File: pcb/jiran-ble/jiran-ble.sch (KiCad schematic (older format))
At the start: 165 parts, among them J1 BATT, J2 USB-C Conn, J3 SWD, J4 BATT, J5 USB-C Conn, J6 SWD, Q1 AO3407, Q3 AO3407, SW1 SW_PUSH, SW10 SW_Push, SW11 SW_Push, SW12 SW_Push, SW13 SW_Push, SW14 SW_Push, SW15 SW_Push, SW16 SW_Push, SW17 SW_Push, SW18 SW_Push, SW19 SW_Push, SW2 SW_Push, SW20 SW_Push, SW21 SW_Push, SW22 SW_Push, SW23 SW_Push, SW24 SW_Push, SW25 SW_Push, SW26 SW_Push, SW27 SW_Push, SW28 SW_Push, SW29 SW_Push, SW3 SW_Push, SW30 SW_PUSH, SW31 SW_Push, SW32 SW_Push, SW33 SW_Push, SW34 SW_Push, SW35 SW_Push, SW36 SW_Push, SW37 SW_Push, SW38 SW_Push, SW39 SW_Push, SW4 SW_Push, SW40 SW_Push, SW41 SW_Push, SW42 SW_Push, SW43 SW_Push, SW44 SW_Push, SW45 SW_Push, SW46 SW_Push, SW47 SW_Push, SW48 SW_Push, SW49 SW_Push, SW5 SW_Push, SW50 SW_Push, SW51 SW_Push, SW52 SW_Push, SW53 SW_Push, SW54 SW_Push, SW55 SW_Push, SW56 SW_Push, SW57 SW_Push, SW58 SW_Push, SW6 SW_Push, SW7 SW_Push, SW8 SW_Push, SW9 SW_Push, U1 XC6220B331MR-G, U3 TP4054, U4 XC6220B331MR-G, U5 E73-2G4M08S1C, U6 TP4054, X2 Crystal

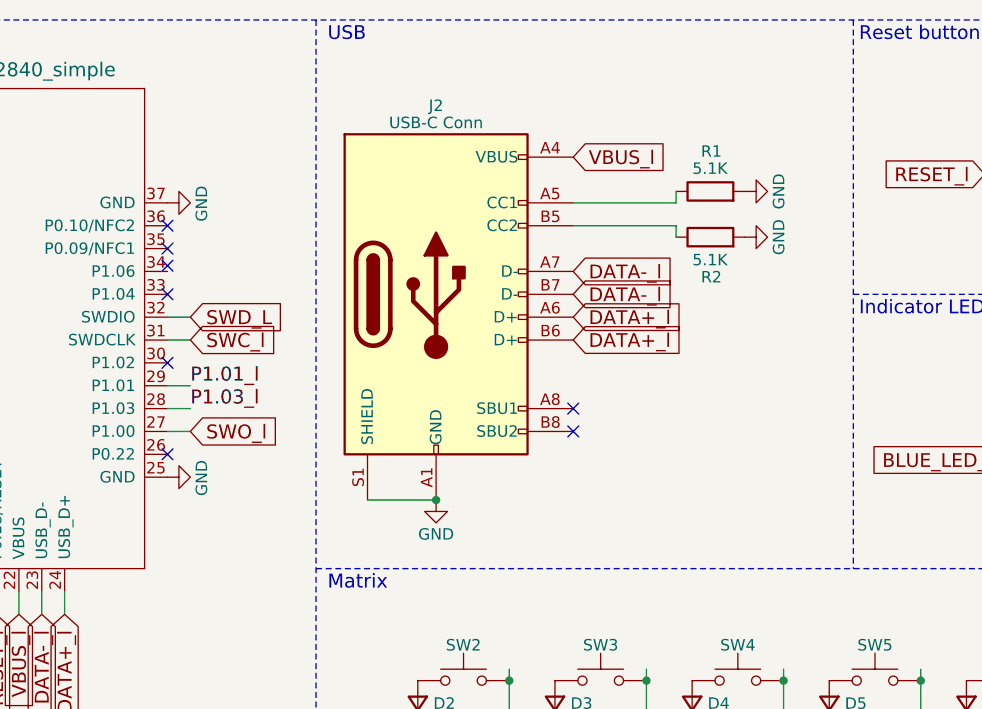
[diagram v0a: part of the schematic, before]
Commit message: USB circuit is now simpler
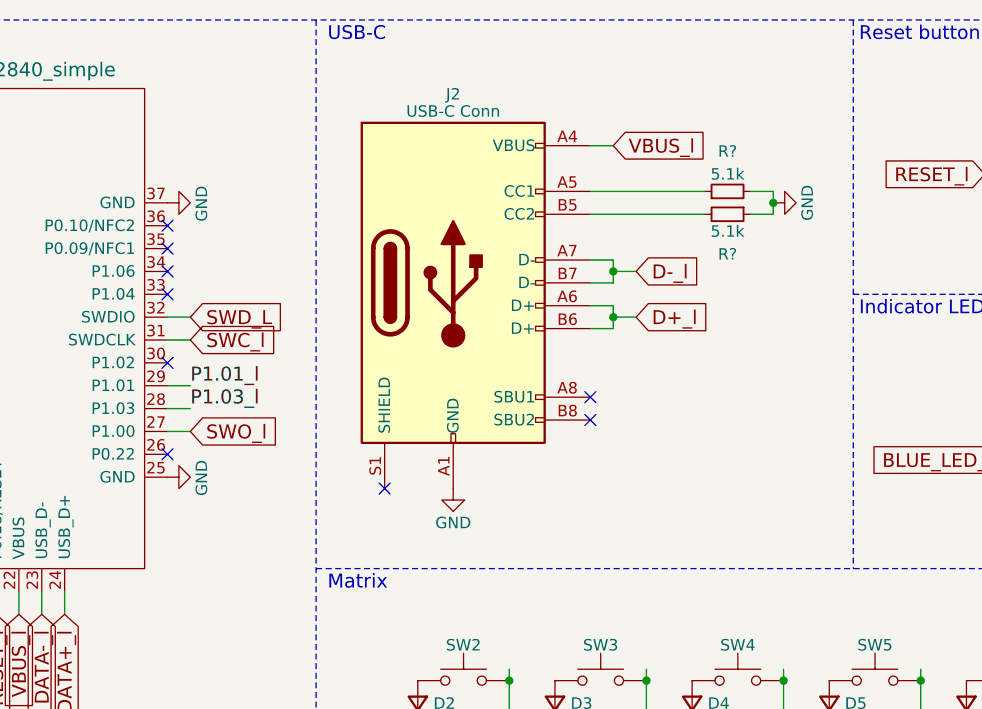
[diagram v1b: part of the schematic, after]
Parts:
- removed R1, R2: 5.1K, jiran-ble:Resistor_SMD_0805, symbol Device:R
- added R? (x2): 5.1k, symbol Device:R_Small
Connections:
- net labels added: D+_l, D-_l
- wire segments 233 -> 245
- no-connect marks 30 -> 31
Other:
- note added: "USB-C"
- moved on the sheet: J2
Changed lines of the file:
@@
 NRF52840
 Text Notes 4100 600  0    60   ~ 0
-USB
+USB-C
 Text Notes 6425 1800 0    60   ~ 0
 Indicator LED
@@
 Text Notes 15415 11075 0    70   ~ 14
 r0.2
-Text GLabel 5175 1600 2    60   Input ~ 0
-DATA-_l
-$Comp
-L Device:R R2
-U 1 1 5CAA680B
-P 5775 1450
-F 0 "R2" V 5600 1400 50  0000 L CNN
-F 1 "5.1K" V 5675 1375 50  0000 L CNN
-F 2 "jiran-ble:Resistor_SMD_0805" V 5705 1450 50  0001 C CNN
-F 3 "~" H 5775 1450 50  0001 C CNN
-	1    5775 1450
-	0    -1   -1   0
-$EndComp
-$Comp
-L Device:R R1
-U 1 1 5CAA879F
-P 5775 1250
-F 0 "R1" V 5950 1200 50  0000 L CNN
-F 1 "5.1K" V 5875 1175 50  0000 L CNN
-F 2 "jiran-ble:Resistor_SMD_0805" V 5705 1250 50  0001 C CNN
-F 3 "~" H 5775 1250 50  0001 C CNN
-	1    5775 1250
-	0    -1   -1   0
-$EndComp
-Text GLabel 5175 1700 2    60   Input ~ 0
-DATA-_l
-Text GLabel 5175 1800 2    60   Input ~ 0
-DATA+_l
-Text GLabel 5175 1900 2    60   Input ~ 0
-DATA+_l
 $Comp
 L power:GND #PWR04
 U 1 1 5E5DBB46
-P 5925 1250
-F 0 "#PWR04" H 5925 1000 50  0001 C CNN
-F 1 "GND" H 5925 1100 50  0000 C CNN
-F 2 "" H 5925 1250 50  0001 C CNN
-F 3 "" H 5925 1250 50  0001 C CNN
-	1    5925 1250
-	0    -1   -1   0
-$EndComp
-$Comp
-L power:GND #PWR06
-U 1 1 5E5DDBCF
-P 5925 1450
-F 0 "#PWR06" H 5925 1200 50  0001 C CNN
-F 1 "GND" H 5925 1300 50  0000 C CNN
-F 2 "" H 5925 1450 50  0001 C CNN
-F 3 "" H 5925 1450 50  0001 C CNN
-	1    5925 1450
+P 6050 1300
+F 0 "#PWR04" H 6050 1050 50  0001 C CNN
+F 1 "GND" H 6050 1150 50  0000 C CNN
+F 2 "" H 6050 1300 50  0001 C CNN
+F 3 "" H 6050 1300 50  0001 C CNN
+	1    6050 1300
 	0    -1   -1   0
 $EndComp
@@
 L power:GND #PWR013
 U 1 1 5E5EC00A
-P 4575 2600
-F 0 "#PWR013" H 4575 2350 50  0001 C CNN
-F 1 "GND" H 4575 2450 50  0000 C CNN
-F 2 "" H 4575 2600 50  0001 C CNN
-F 3 "" H 4575 2600 50  0001 C CNN
-	1    4575 2600
+P 4650 2550
+F 0 "#PWR013" H 4650 2300 50  0001 C CNN
+F 1 "GND" H 4650 2400 50  0000 C CNN
+F 2 "" H 4650 2550 50  0001 C CNN
+F 3 "" H 4650 2550 50  0001 C CNN
+	1    4650 2550
 	1    0    0    -1
 $EndComp
-Text GLabel 5175 1100 2    60   Input ~ 0
+Text GLabel 5350 1050 2    60   Input ~ 0
 VBUS_l
 $Comp
 L nrfmicro-rescue:USB_C_Receptacle_USB2.0-Connector J2
 U 1 1 5C743564
-P 4575 1700
-F 0 "J2" H 4575 2525 50  0000 C CNN
-F 1 "USB-C Conn" H 4575 2450 50  0000 C CNN
-F 2 "jiran-ble:USB-C_MidMount" H 4682 2475 50  0001 C CNN
-F 3 "https://www.usb.org/sites/default/files/documents/usb_type-c.zip" H 4725 1700 50  0001 C CNN
-	1    4575 1700
+P 4650 1650
+F 0 "J2" H 4650 2475 50  0000 C CNN
+F 1 "USB-C Conn" H 4650 2400 50  0000 C CNN
+F 2 "jiran-ble:USB-C_MidMount" H 4757 2425 50  0001 C CNN
+F 3 "https://www.usb.org/sites/default/files/documents/usb_type-c.zip" H 4800 1650 50  0001 C CNN
+	1    4650 1650
 	1    0    0    -1
 $EndComp
@@
 Connection ~ 1075 4550
 Wire Wire Line
-	4275 2600 4575 2600
-Connection ~ 4575 2600
-Wire Wire Line
 	1675 4950 1725 4950
 Wire Wire Line
@@
 Wire Wire Line
 	11825 2050 11925 2050
-NoConn ~ 5175 2200
-NoConn ~ 5175 2300
+NoConn ~ 5250 2150
+NoConn ~ 5250 2250
 Text Notes 3175 4700 0    60   ~ 0
 RProg\n10k\n5k\n2.5k\n2k\n1.25k
@@
 Text Notes 3075 4075 0    60   ~ 0
 RProg = 1000/IBat\nIBat in amps
-Wire Wire Line
-	5175 1300 5625 1300
-Wire Wire Line
-	5625 1300 5625 1250
-Wire Wire Line
-	5175 1400 5625 1400
-Wire Wire Line
-	5625 1400 5625 1450
 Text GLabel 8775 2325 0    60   Input ~ 0
 nRF_VDD_l
@@
 NoConn ~ 3400 2000
 NoConn ~ 3400 1700
-NoConn ~ 3400 1575
+NoConn ~ 3400 1600
 NoConn ~ 3400 1500
 NoConn ~ 3400 1400
 NoConn ~ 1500 1600
 NoConn ~ 1500 1700
+$Comp
+L Device:R_Small R?
+U 1 1 609F1795
+P 5850 1250
+F 0 "R?" V 6025 1250 50  0000 C CNN
+F 1 "5.1k" V 5925 1250 50  0000 C CNN
+F 2 "" H 5850 1250 50  0001 C CNN
+F 3 "~" H 5850 1250 50  0001 C CNN
+	1    5850 1250
+	0    -1   -1   0
+$EndComp
+$Comp
+L Device:R_Small R?
+U 1 1 609F2B00
+P 5850 1350
+F 0 "R?" V 6025 1350 50  0000 C CNN
+F 1 "5.1k" V 5925 1350 50  0000 C CNN
+F 2 "" H 5850 1350 50  0001 C CNN
+F 3 "~" H 5850 1350 50  0001 C CNN
+	1    5850 1350
+	0    1    1    0
+$EndComp
+Text GLabel 5450 1600 2    61   Input ~ 0
+D-_l
+Wire Wire Line
+	5250 1550 5350 1550
+Wire Wire Line
+	5350 1650 5250 1650
+Wire Wire Line
+	5350 1550 5350 1600
+Wire Wire Line
+	5450 1600 5350 1600
+Connection ~ 5350 1600
+Wire Wire Line
+	5350 1600 5350 1650
+Text GLabel 5450 1800 2    61   Input ~ 0
+D+_l
+Wire Wire Line
+	5250 1750 5350 1750
+Wire Wire Line
+	5350 1850 5250 1850
+Wire Wire Line
+	5350 1750 5350 1800
+Wire Wire Line
+	5450 1800 5350 1800
+Connection ~ 5350 1800
+Wire Wire Line
+	5350 1800 5350 1850
+Wire Wire Line
+	5350 1050 5250 1050
+Wire Wire Line
+	5750 1350 5250 1350
+Wire Wire Line
+	5750 1250 5250 1250
+Wire Wire Line
+	5950 1250 6050 1250
+Wire Wire Line
+	6050 1350 5950 1350
+NoConn ~ 4350 2550
+Wire Wire Line
+	6050 1250 6050 1300
+Connection ~ 6050 1300
+Wire Wire Line
+	6050 1300 6050 1350
 $EndSCHEMATC
